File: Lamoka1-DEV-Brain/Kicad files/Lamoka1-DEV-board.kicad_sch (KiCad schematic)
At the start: 50 parts, among them J1 Conn_01x13_Pin, J3 USB_C_Receptacle_USB2.0_14P, SW1 PTS636 SM43J SMTR LFS, U1 RP2354A, U2 AMS1117-3.3, U3 74AHCT1G125, X1 ABM8-272-T3

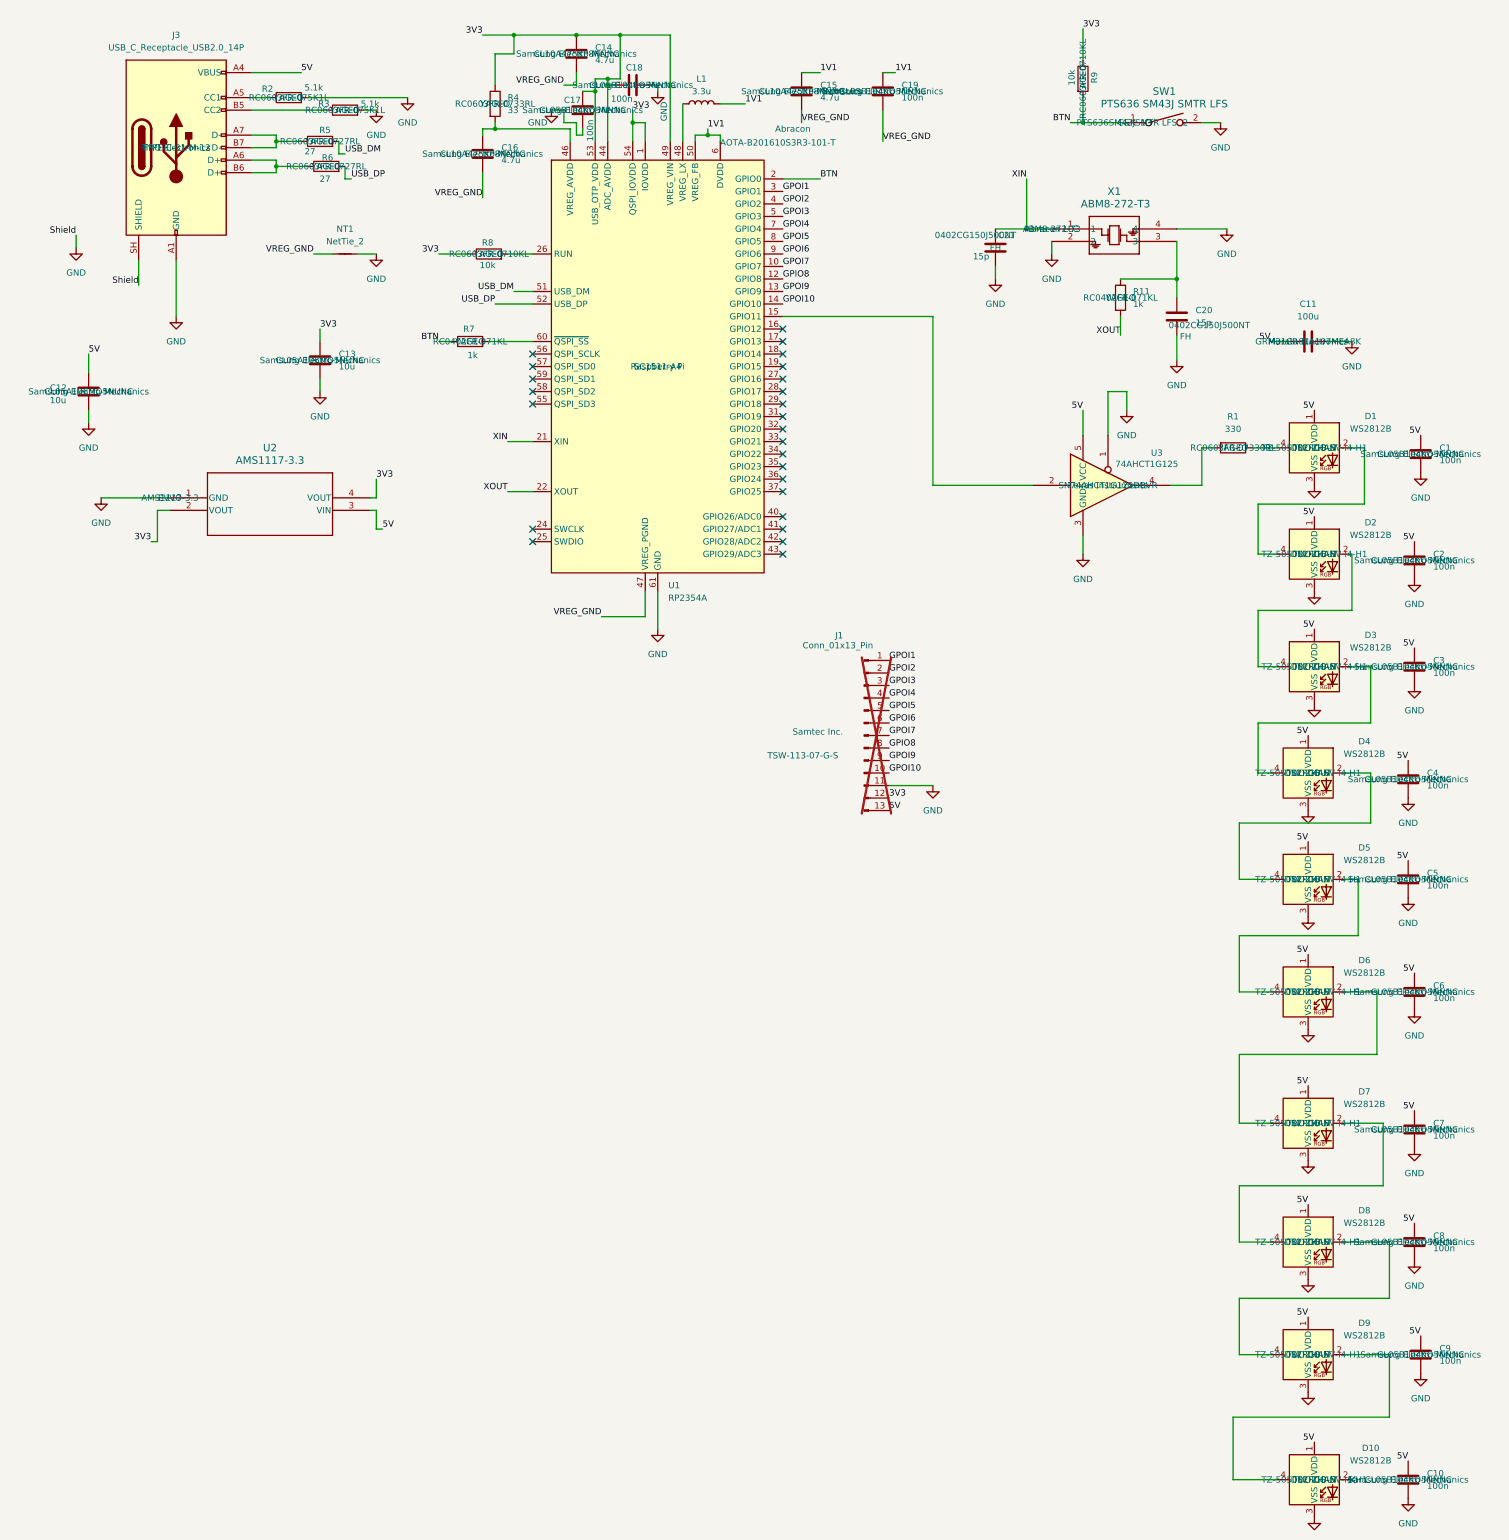
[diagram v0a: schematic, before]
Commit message: Cleaning up the DEV-Brains folder
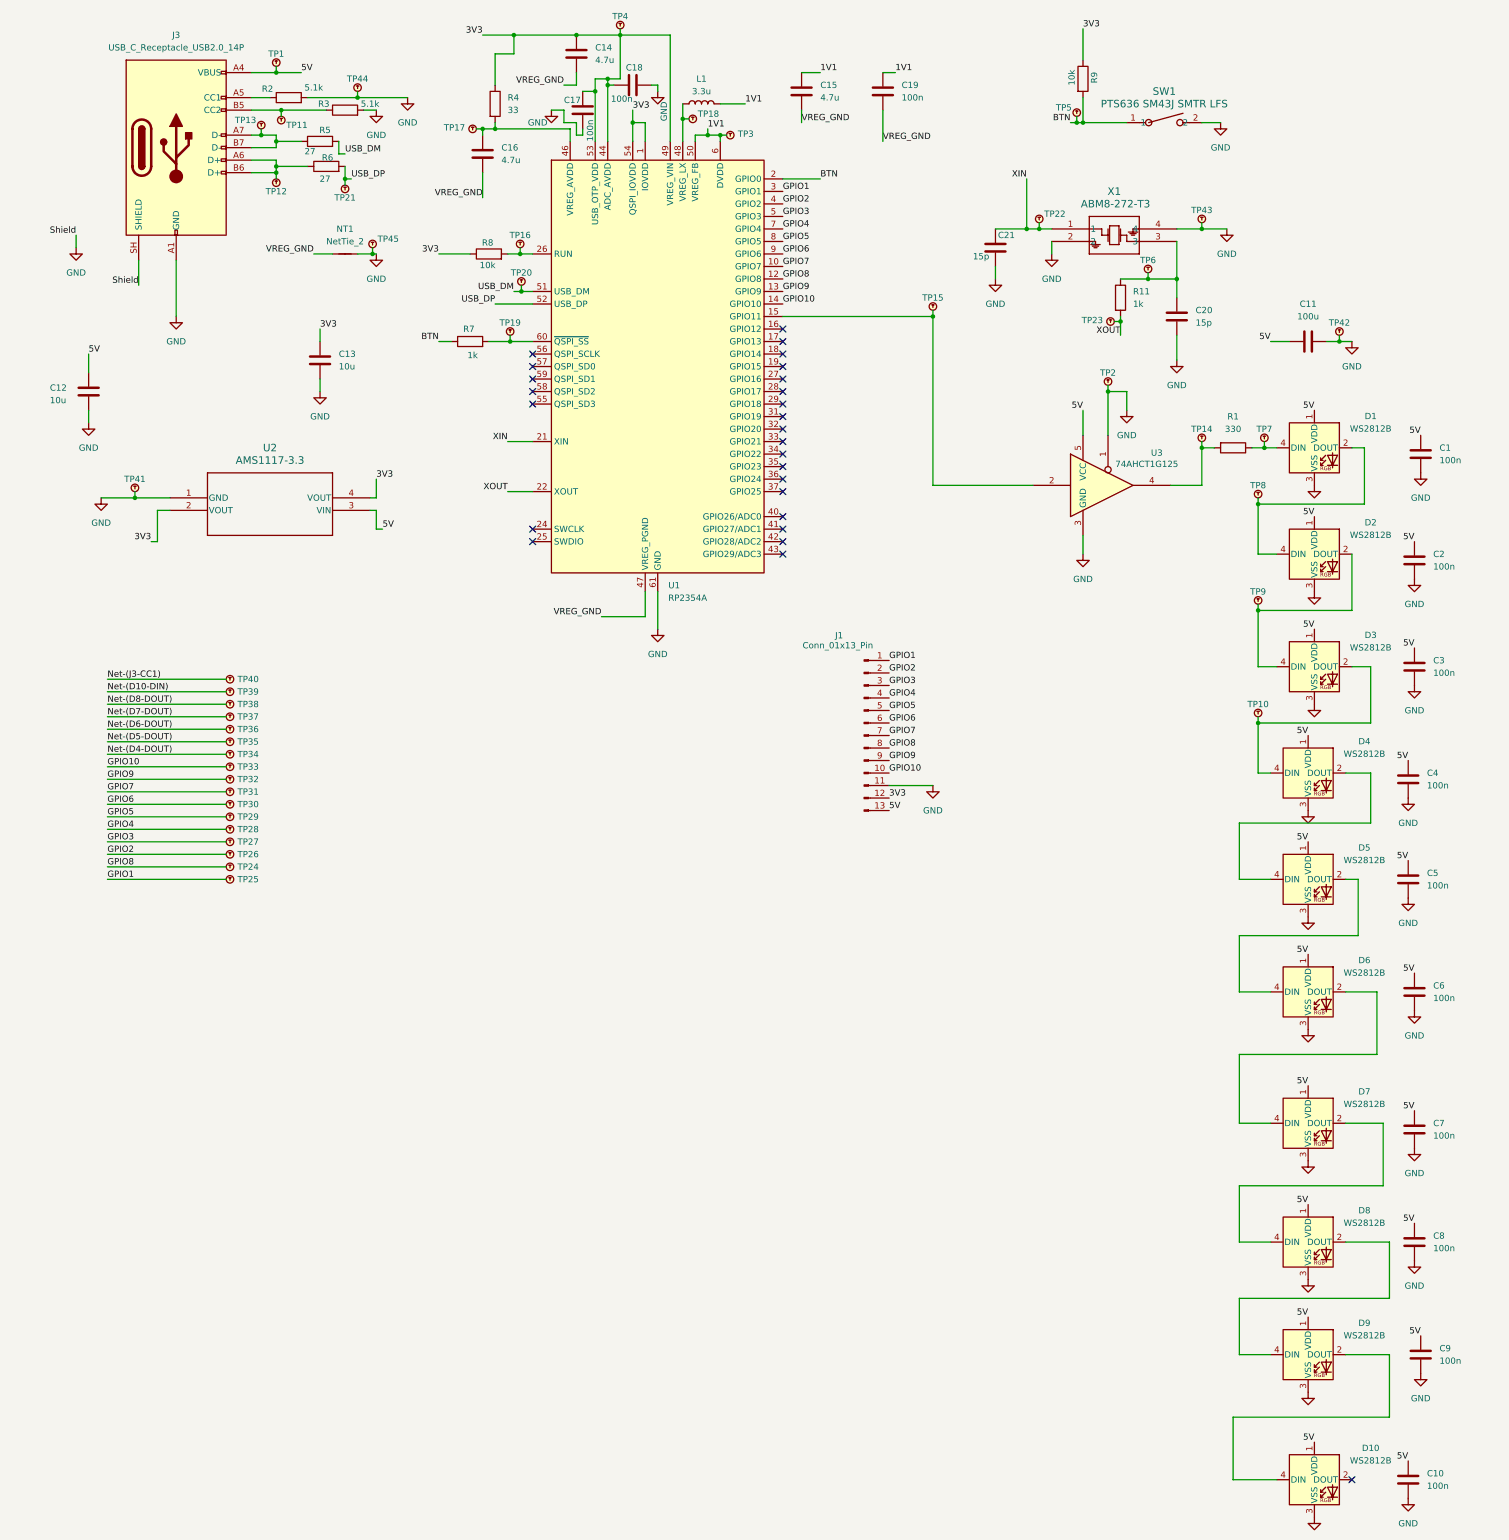
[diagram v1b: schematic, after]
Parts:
- added TP1, TP10, TP13, TP14, TP15, TP16, TP19, TP2, TP20, TP22, TP4, TP41, TP42, TP43, TP44, TP45, TP5, TP6, TP7, TP8, TP9: Tomachie_TP_N, Pads:TPS127, symbol Pads:Tomachie_TP_N
- added TP11, TP12, TP21: Tomachie_TP_S, Pads:TPS127, symbol Pads:Tomachie_TP_S
- added TP17, TP23: Tomachie_TP_W, Pads:TPS127, symbol Pads:Tomachie_TP_W
- added TP18, TP24, TP25, TP26, TP27, TP28, TP29, TP3, TP30, TP31, TP32, TP33, TP34, TP35, TP36, TP37, TP38, TP39, TP40: Tomachie_TP_E, Pads:TPS127, symbol Pads:Tomachie_TP_E
- J1: now fitted
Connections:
- net 1V1: now also TP3.1
- net 3V3: now also TP4.1
- net 5V: now also TP1.1
- net BTN: now also TP5.1
- net GND: now also TP2.1, TP41.1, TP42.1, TP43.1, TP44.1, TP45.1
- net GPIO8: now also TP24.1
- net USB_DM: now also TP20.1
- net USB_DP: now also TP21.1
- net XIN: now also TP22.1
- net XOUT: now also TP23.1
- net at J3.A6 (D+), J3.B6 (D+), R6.1: now also TP12.1
- net at J3.A7 (D-), J3.B7 (D-), R5.1: now also TP13.1
- net at J3.B5 (CC2), R3.1: now also TP11.1
- net at D3.2 (DOUT), D4.4 (DIN): now also TP10.1
- net at D2.2 (DOUT), D3.4 (DIN): now also TP9.1
- net at L1.1, U1.48 (VREG_LX): now also TP18.1
- net at D1.2 (DOUT), D2.4 (DIN): now also TP8.1
- net at R8.2, U1.26 (RUN): now also TP16.1
- net at D1.4 (DIN), R1.1: now also TP7.1
- net at R1.2, U3.4: now also TP14.1
- net at R7.2, U1.60 (~{QSPI_SS}): now also TP19.1
- net at U1.15 (GPIO11), U3.2: now also TP15.1
- net at C16.1, R4.2, U1.46 (VREG_AVDD): now also TP17.1
- net at C20.1, R11.1, X1.3: now also TP6.1
- net GPOI1 renamed GPIO1
- net GPIO1: now also TP25.1
- net GPOI10 renamed GPIO10
- net GPIO10: now also TP33.1
- net GPOI2 renamed GPIO2
- net GPIO2: now also TP26.1
- net GPOI3 renamed GPIO3
- net GPIO3: now also TP27.1
- net GPOI4 renamed GPIO4
- net GPIO4: now also TP28.1
- net GPOI5 renamed GPIO5
- net GPIO5: now also TP29.1
- net GPOI6 renamed GPIO6
- net GPIO6: now also TP30.1
- net GPOI7 renamed GPIO7
- net GPIO7: now also TP31.1
- net GPOI9 renamed GPIO9
- net GPIO9: now also TP32.1
- new net Net-(D10-DIN): TP39.1
- new net Net-(D4-DOUT): TP34.1
- new net Net-(D5-DOUT): TP35.1
- new net Net-(D6-DOUT): TP36.1
- new net Net-(D7-DOUT): TP37.1
- new net Net-(D8-DOUT): TP38.1
- new net Net-(J3-CC1): TP40.1
